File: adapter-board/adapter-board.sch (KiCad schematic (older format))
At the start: 18 parts, among them J1 TAPE, J2 Conn_01x02_Female, J3 HEADER3, J4 HEADER1, J5 BLU, J6 SOP16, J7 HEADER4, J8 HEADER2, J9 Conn_01x05_Female

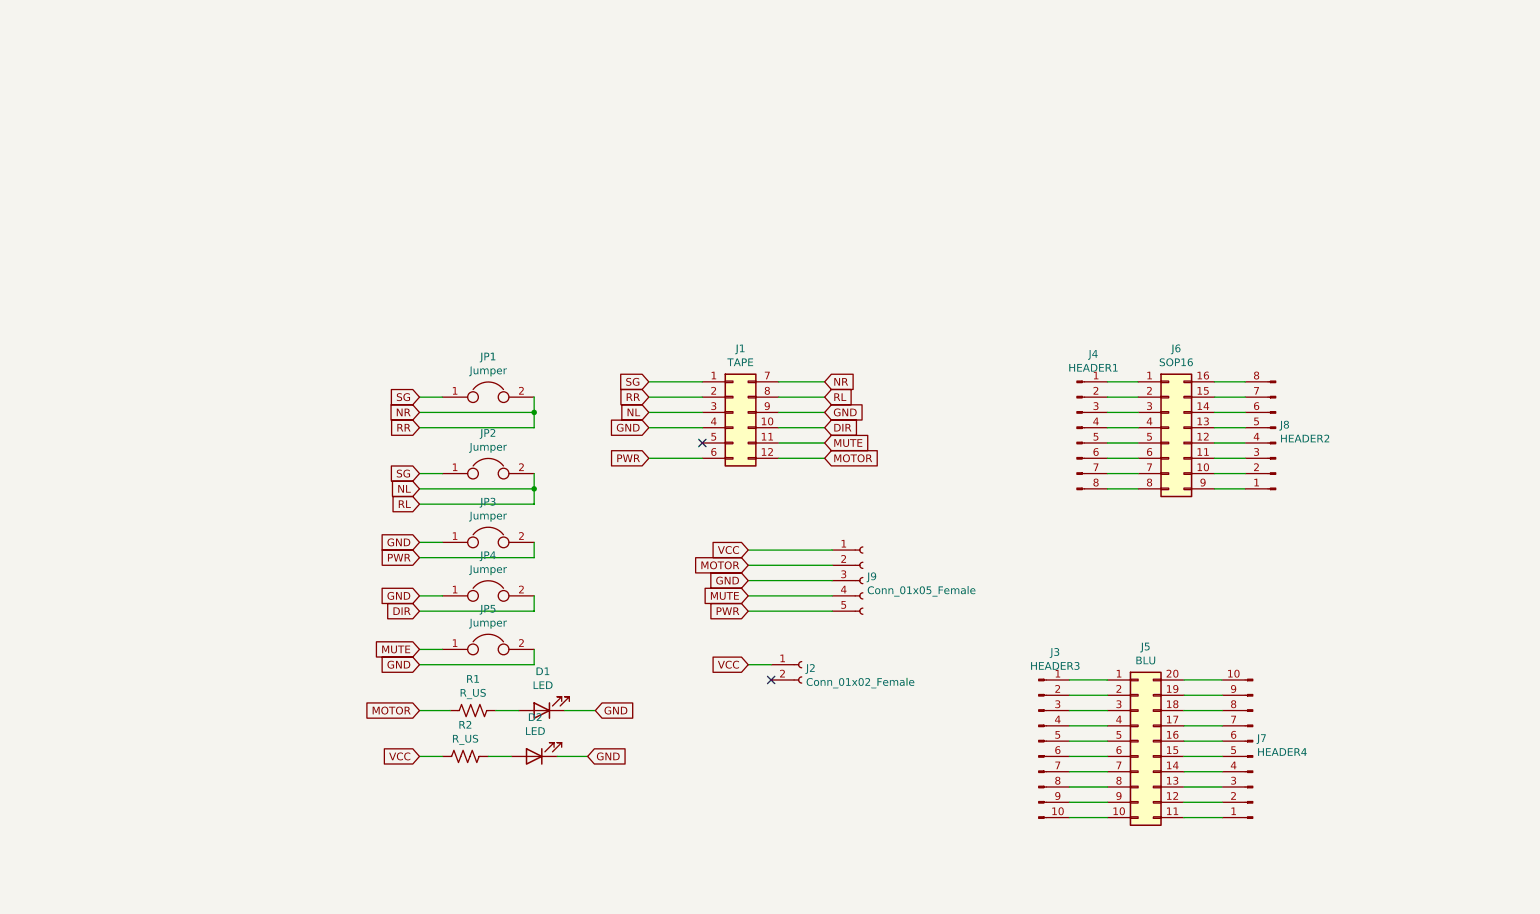
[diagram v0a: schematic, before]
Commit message: sync
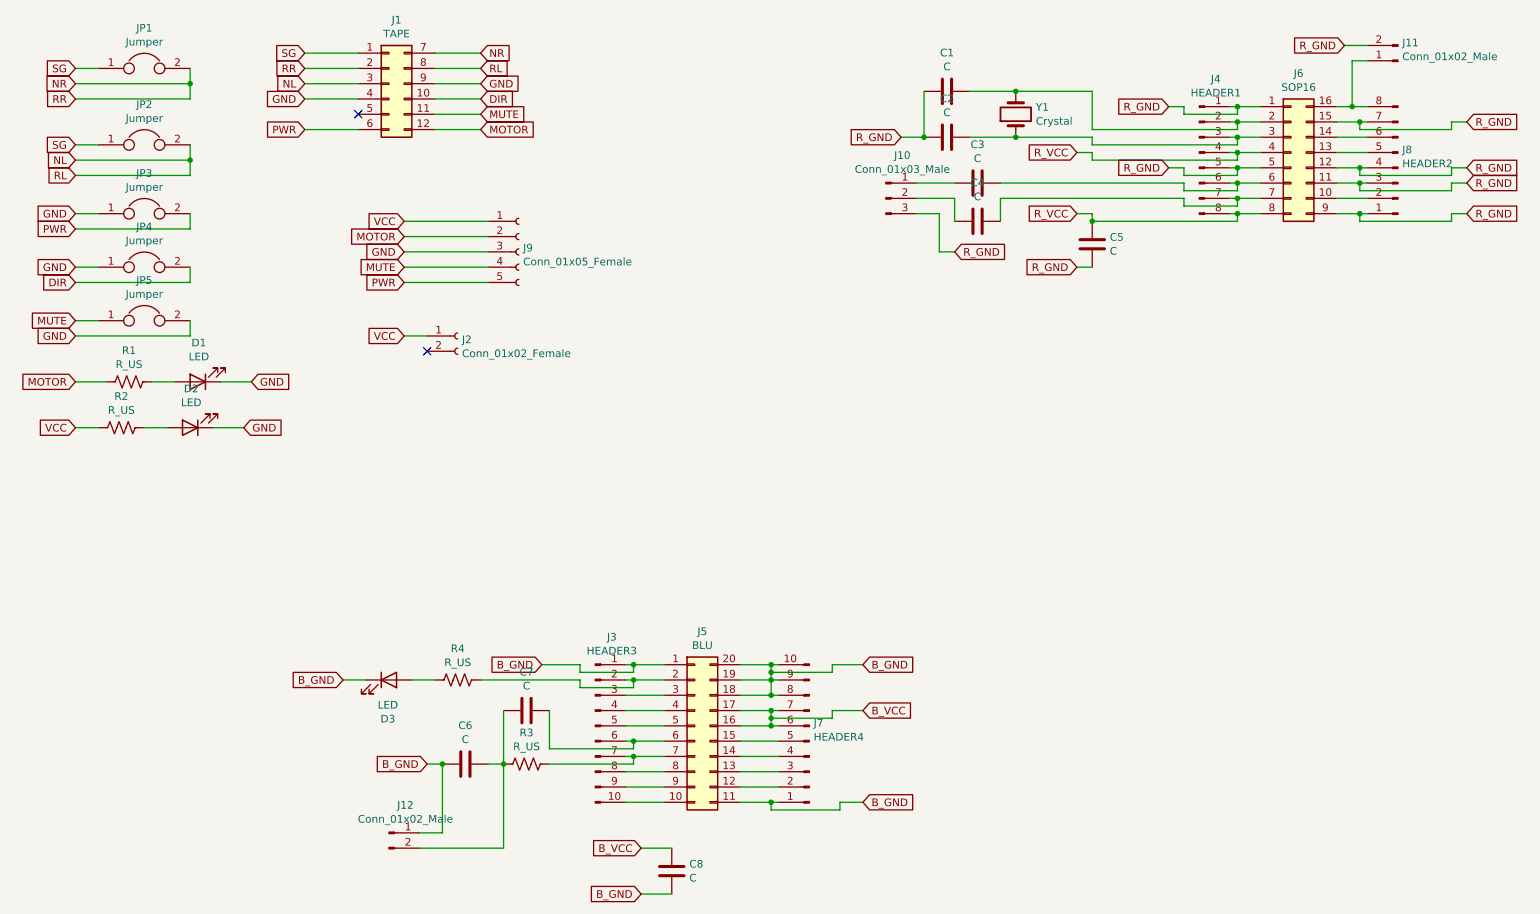
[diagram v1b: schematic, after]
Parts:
- added C1, C2, C3, C4, C5, C6, C7, C8: C, Capacitor_SMD:C_0805_2012Metric_Pad1.18x1.45mm_HandSolder, symbol Device:C
- added D3: LED, LED_SMD:LED_0805_2012Metric_Pad1.15x1.40mm_HandSolder, symbol Device:LED
- added J10: Conn_01x03_Male, Connector_PinHeader_2.54mm:PinHeader_1x03_P2.54mm_Vertical, symbol Connector:Conn_01x03_Male
- added J11, J12: Conn_01x02_Male, Connector_PinHeader_2.54mm:PinHeader_1x02_P2.54mm_Vertical, symbol Connector:Conn_01x02_Male
- added R3, R4: R_US, Resistor_SMD:R_0805_2012Metric_Pad1.20x1.40mm_HandSolder, symbol Device:R_US
- added Y1: Crystal, Crystal:Crystal_C38-LF_D3.0mm_L8.0mm_Horizontal_1EP_style1, symbol Device:Crystal
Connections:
- net R_GND: now reaches J4.1 (Pin_1), J6.1 (Pin_1)
- net R_GND: now also J4.5 (Pin_5), J6.11 (Pin_11), J6.12 (Pin_12), J6.15 (Pin_15), J6.5 (Pin_5), J6.9 (Pin_9), J8.1 (Pin_1), J8.3 (Pin_3), J8.4 (Pin_4), J8.7 (Pin_7), C1.2, C2.2, C5.1, J10.3 (Pin_3), J11.2 (Pin_2)
- net at J6.16 (Pin_16), J8.8 (Pin_8): now also J11.1 (Pin_1)
- net at J4.2 (Pin_2), J6.2 (Pin_2): now also C1.1, Y1.2
- net at J4.3 (Pin_3), J6.3 (Pin_3): now also C2.1, Y1.1
- net R_VCC: now reaches J4.4 (Pin_4), J6.4 (Pin_4)
- net R_VCC: now also J4.8 (Pin_8), J6.8 (Pin_8), C5.2
- net at J4.6 (Pin_6), J6.6 (Pin_6): now also C3.1
- net at J4.7 (Pin_7), J6.7 (Pin_7): now also C4.1
- net B_GND: now reaches J3.1 (Pin_1), J5.1 (Pin_1)
- net B_GND: now also J5.11 (Pin_11), J5.18 (Pin_18), J5.19 (Pin_19), J5.20 (Pin_20), J7.1 (Pin_1), J7.10 (Pin_10), J7.8 (Pin_8), J7.9 (Pin_9), C6.1, C8.1, D3.1 (K), J12.1 (Pin_1)
- net B_VCC: now reaches J5.16 (Pin_16), J7.6 (Pin_6)
- net B_VCC: now also J5.17 (Pin_17), J7.7 (Pin_7), C8.2
- net at J3.2 (Pin_2), J5.2 (Pin_2): now also R4.1
- net at J3.6 (Pin_6), J5.6 (Pin_6): now also C7.1
- net at J3.7 (Pin_7), J5.7 (Pin_7): now also R3.1
- new net: C3.2, J10.1 (Pin_1)
- new net: C4.2, J10.2 (Pin_2)
- new net: C6.2, C7.2, J12.2 (Pin_2), R3.2
- new net: D3.2 (A), R4.2
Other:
- moved on the sheet: D1, D2, J1, J2, J3, J4, J5, J6, J7, J8, J9, JP1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
